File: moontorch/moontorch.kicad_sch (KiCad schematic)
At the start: 32 parts, among them J2 Pogo_VLED_1, J3 Pogo_VLED_2, J4 BAT, J5 Torchbutton, J6 UART, J7 USB, J8 Pogo_GND, Q1 AP2317SD, SW3 RESET, SW4 BOOT, U1 HT-CT62, U2 L80-R, U3 XTX XTP2038-330AS2CT, U4 2.4GHz

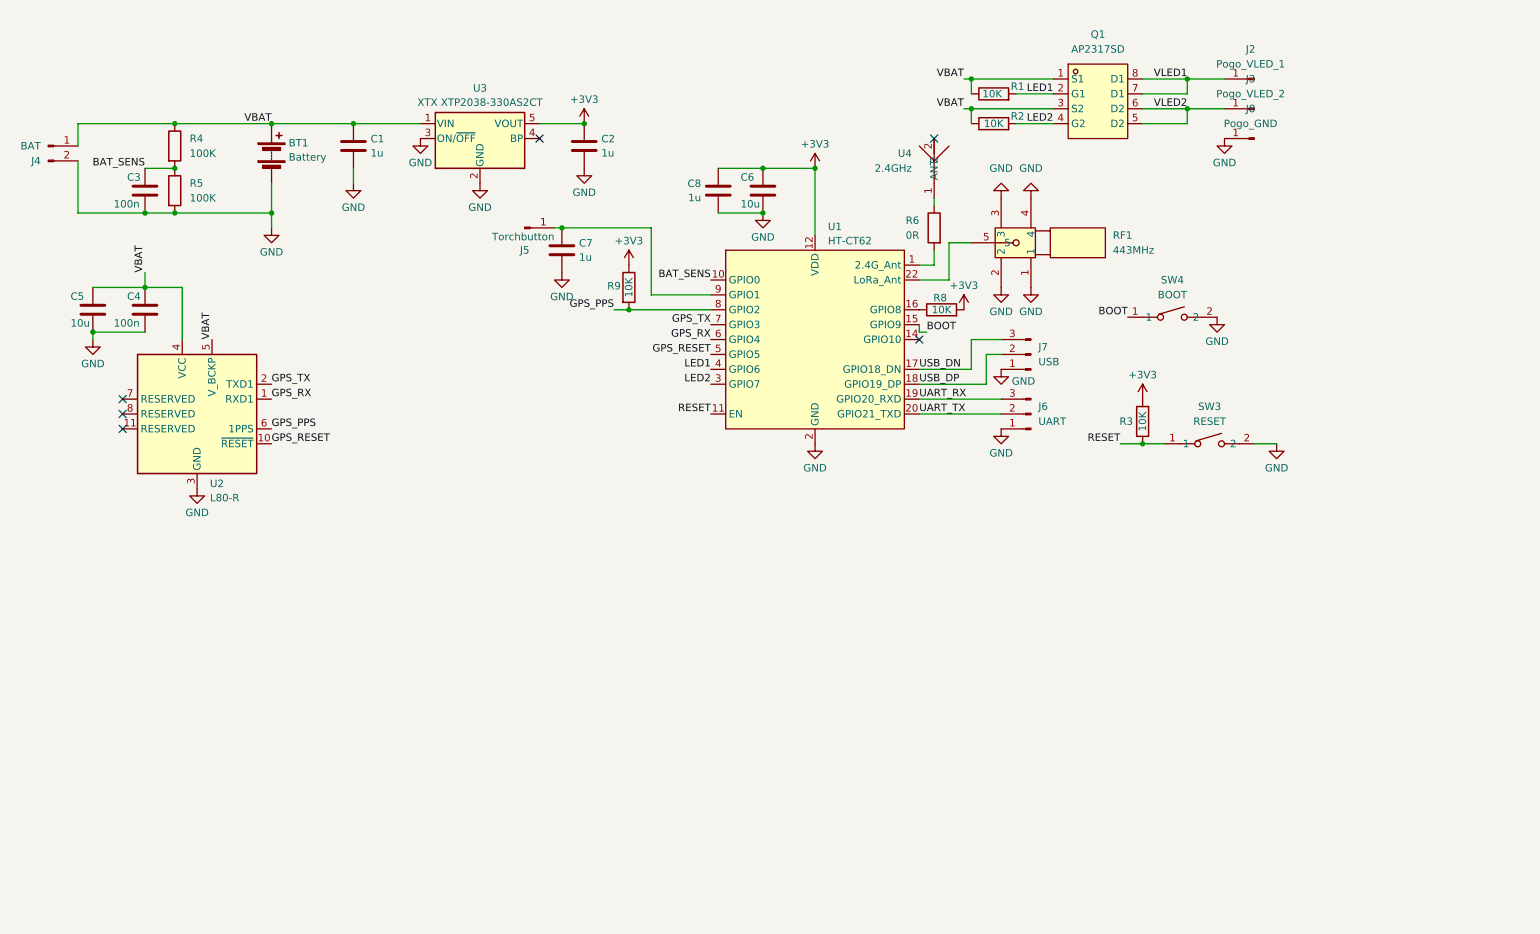
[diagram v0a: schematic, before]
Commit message: zwischenstand bestellfähig 1
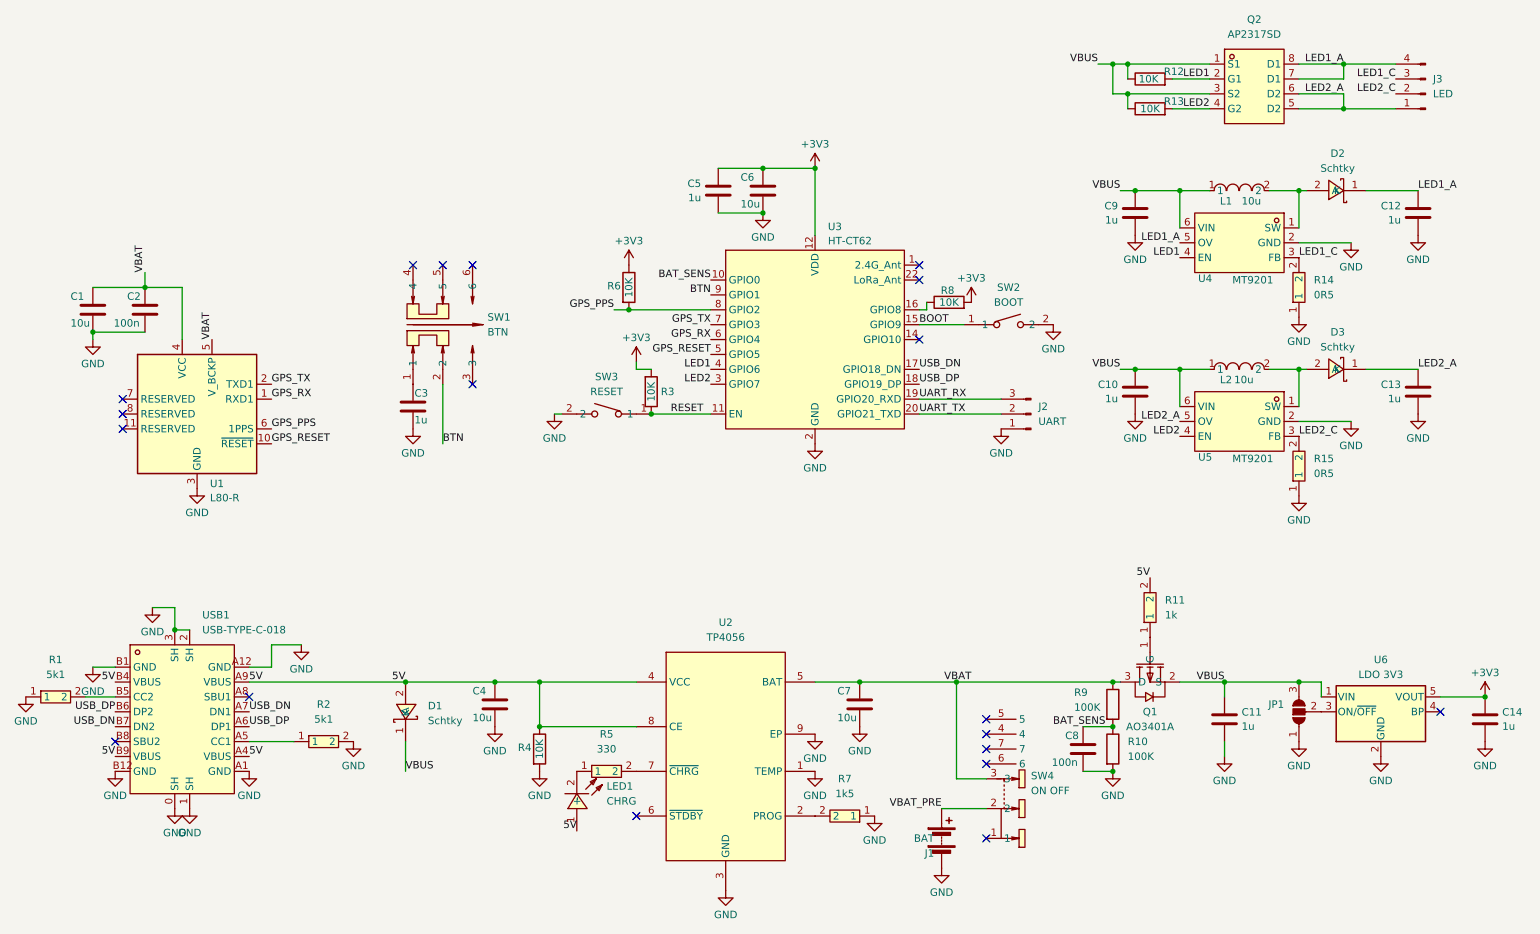
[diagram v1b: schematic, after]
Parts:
- removed BT1: Battery, hacrafu:Battery 230525, symbol Device:Battery
- removed J2: Pogo_VLED_1, hacrafu:Pogo Pin 3015, symbol Connector:Conn_01x01_Pin
- removed J3: Pogo_VLED_2, hacrafu:Pogo Pin 3015, symbol Connector:Conn_01x01_Pin
- removed J5: Torchbutton, hacrafu:Tochbutton GND, symbol Connector:Conn_01x01_Pin
- removed J7: USB, Connector_PinHeader_2.54mm:PinHeader_1x03_P2.54mm_Vertical, symbol Connector:Conn_01x03_Pin
- removed J8: Pogo_GND, hacrafu:Pogo Pin 3015, symbol Connector:Conn_01x01_Pin
- removed R6: 0R, Resistor_SMD:R_0603_1608Metric_Pad0.98x0.95mm_HandSolder, symbol Device:R
- removed RF1: 443MHz, EasyEDA:SMA-SMD_BWSMA-KE-P001, symbol EasyEDA:HJ-SMA275
- removed U4: 2.4GHz, EasyEDA:ANT-SMD_L5.0-W2.0, symbol EasyEDA:2450AT42A100E
- added C10, C12, C13, C9: 1u, Capacitor_SMD:C_0603_1608Metric_Pad1.08x0.95mm_HandSolder, symbol Device:C
- added C4, C7: 10u, Capacitor_SMD:C_0603_1608Metric_Pad1.08x0.95mm_HandSolder, symbol Device:C
- added D1, D2, D3: Schtky, EasyEDA:SOD-323_L1.8-W1.3-LS2.5-RD, symbol EasyEDA:1N5819WS
- added J3: LED, Connector_PinHeader_2.54mm:PinHeader_1x04_P2.54mm_Vertical, symbol Connector:Conn_01x04_Pin
- added JP1: SolderJumper_3_Open, Jumper:SolderJumper-3_P1.3mm_Open_Pad1.0x1.5mm, symbol Jumper:SolderJumper_3_Open
- added L1, L2: 10u, EasyEDA:IND-SMD_L5.4-W5.2_FXL0530, symbol EasyEDA:FXL0530-100-M
- added LED1: CHRG, LED_SMD:LED_0805_2012Metric_Pad1.15x1.40mm_HandSolder, symbol EasyEDA:17-21SUYC_TR8
- added Q1: AO3401A, EasyEDA:SOT-23_L2.9-W1.3-P1.90-LS2.4-BR, symbol EasyEDA:AO3401A
- added R1, R2: 5k1, Resistor_SMD:R_0603_1608Metric_Pad0.98x0.95mm_HandSolder, symbol EasyEDA:0603WAF5101T5E
- added R11: 1k, Resistor_SMD:R_0603_1608Metric_Pad0.98x0.95mm_HandSolder, symbol EasyEDA:0603WAF1001T5E
- added R14, R15: 0R5, Resistor_SMD:R_1206_3216Metric_Pad1.30x1.75mm_HandSolder, symbol EasyEDA:1206W4F500LT5E
- added R4: 10K, Resistor_SMD:R_0603_1608Metric_Pad0.98x0.95mm_HandSolder, symbol Device:R
- added R5: 330, Resistor_SMD:R_0603_1608Metric_Pad0.98x0.95mm_HandSolder, symbol EasyEDA:0603WAF3300T5E
- added R7: 1k5, Resistor_SMD:R_0603_1608Metric_Pad0.98x0.95mm_HandSolder, symbol EasyEDA:0603WAF1501T5E
- added SW1: BTN, EasyEDA:SW-SMD_6P-L5.8-W5.8-P2.00-LS8.5-TR, symbol EasyEDA:XKB5858-Z-TP_C840833
- added SW4: ON OFF, EasyEDA:SW-TH_K3-1296S-E1, symbol EasyEDA:K3-1296S-E1_C128955
- added U2: TP4056, EasyEDA:ESOP-8_L4.9-W3.9-P1.27-LS6.0-BL-EP, symbol EasyEDA:TP4056
- added U4, U5: MT9201, EasyEDA:SOT-23-6_L2.9-W1.6-P0.95-LS2.8-BR, symbol EasyEDA:MT9201
- added USB1: USB-TYPE-C-018, EasyEDA:USB-C_SMD-TYPE-C-31-M-12, symbol EasyEDA:USB-TYPE-C-018
- J1: renamed from J4; footprint Connector_PinHeader_2.54mm:PinHeader_1x02_P2.54mm_Horizontal -> hacrafu:Battery 230525; symbol Connector:Conn_01x02_Pin -> Device:Battery
- U6: renamed from U3; value XTX XTP2038-330AS2CT -> LDO 3V3
- renumbered C5 to C1, C1 to C11, C2 to C14, C4 to C2, C7 to C3, C8 to C5, C3 to C8, J6 to J2, Q1 to Q2, R5 to R10, R1 to R12, R2 to R13, R9 to R6, R4 to R9, SW4 to SW2, U2 to U1, U1 to U3
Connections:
- net GND: now also C10.2, C12.2, C13.2, C4.2, C7.2, C9.2, JP1.1 (A), R1.1, R14.1, R15.1, R2.2, R4.2, R7.1, U2.1 (TEMP), U2.3 (GND), U2.9 (EP), U4.2 (GND), U5.2 (GND), USB1.0 (SH), USB1.1 (SH), USB1.2 (SH), USB1.3 (SH), USB1.A1 (GND), USB1.A12 (GND), USB1.B1 (GND), USB1.B12 (GND); no longer U6.3 (ON/~{OFF})
- net LED1: now also U4.4 (EN)
- net LED2: now also U5.4 (EN)
- net USB_DN: now also USB1.A7 (DN1), USB1.B7 (DN2)
- net USB_DP: now also USB1.A6 (DP1), USB1.B6 (DP2)
- net VBAT: now also C7.1, Q1.3 (D), SW4.3, U2.5 (BAT); no longer C11.1, J1.1 (Pin_1), Q2.1 (S1), Q2.3 (S2), R12.1, R13.1, U6.1 (VIN)
- net at C3.1: now also SW1.1; no longer U3.9 (GPIO1)
- net VLED1 renamed LED1_A
- net LED1_A: now also C12.1, D2.1 (K), J3.4 (Pin_4), U4.5 (OV)
- net VLED2 renamed LED2_A
- net LED2_A: now also C13.1, D3.1 (K), J3.1 (Pin_1), U5.5 (OV)
- new net: D2.2 (A), L1.2, U4.1 (SW)
- new net: R7.2, U2.2 (PROG)
- new net: R5.2, U2.7 (~{CHRG})
- new net: LED1.2 (-), R5.1
- new net: D3.2 (A), L2.2, U5.1 (SW)
- new net: R2.1, USB1.A5 (CC1)
- new net: R1.2, USB1.B5 (CC2)
- new net: Q1.1 (G), R11.1
- new net: JP1.2 (C), U6.3 (ON/~{OFF})
- new net 5V: C4.1, D1.2 (A), LED1.1 (+), R11.2, R4.1, U2.4 (VCC), U2.8 (CE), USB1.A4 (VBUS), USB1.A9 (VBUS), USB1.B4 (VBUS), USB1.B9 (VBUS)
- new net BTN: SW1.2, U3.9 (GPIO1)
- new net LED1_C: J3.3 (Pin_3), R14.2, U4.3 (FB)
- new net LED2_C: J3.2 (Pin_2), R15.2, U5.3 (FB)
- new net VBAT_PRE: J1.1 (+), SW4.2
- new net VBUS: C10.1, C11.1, C9.1, D1.1 (K), JP1.3 (B), L1.1, L2.1, Q1.2 (S), Q2.1 (S1), Q2.3 (S2), R12.1, R13.1, U4.6 (VIN), U5.6 (VIN), U6.1 (VIN)
- no-connect marks 6 -> 19
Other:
- moved on the sheet: C11, C14, C3, C8, Q2, R10, R12, R13, R3, R8, R9, SW2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
